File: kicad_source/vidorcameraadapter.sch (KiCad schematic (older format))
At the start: 67 parts, among them CN1 TE_2041119-2, CN2 RS2-20-G, CN3 DNI, U1 SN74LVC2G34DBV

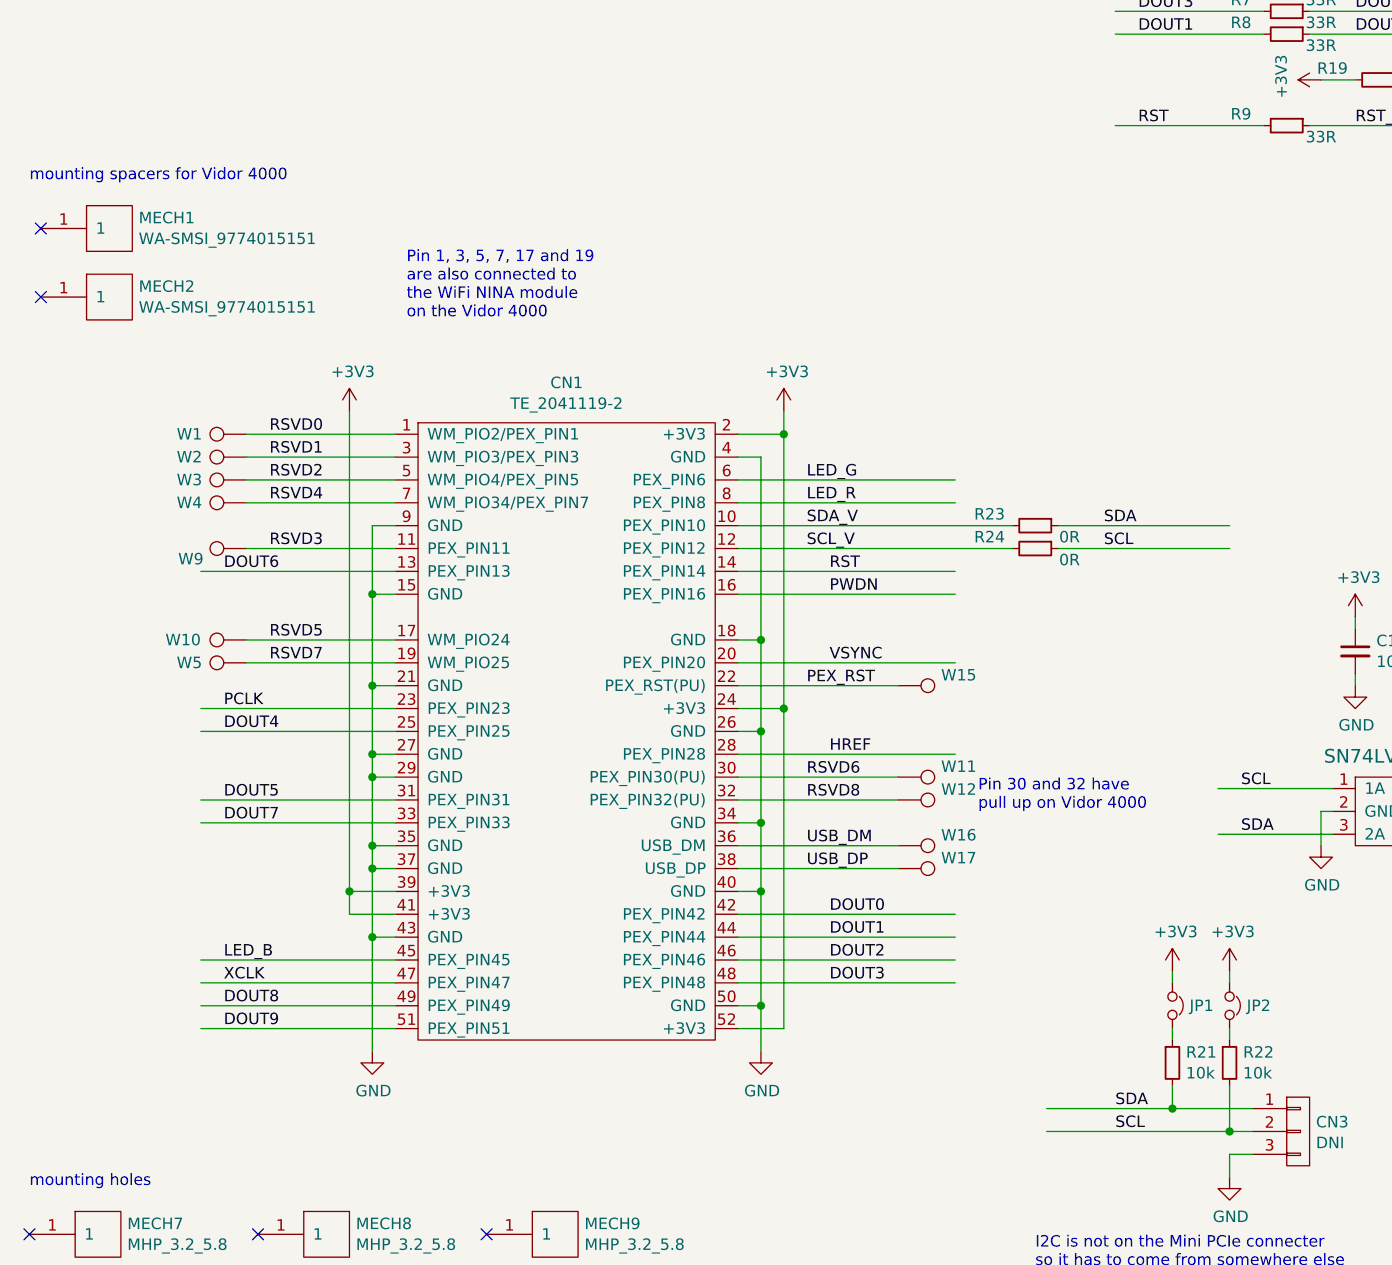
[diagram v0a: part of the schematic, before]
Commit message: restored design files from master
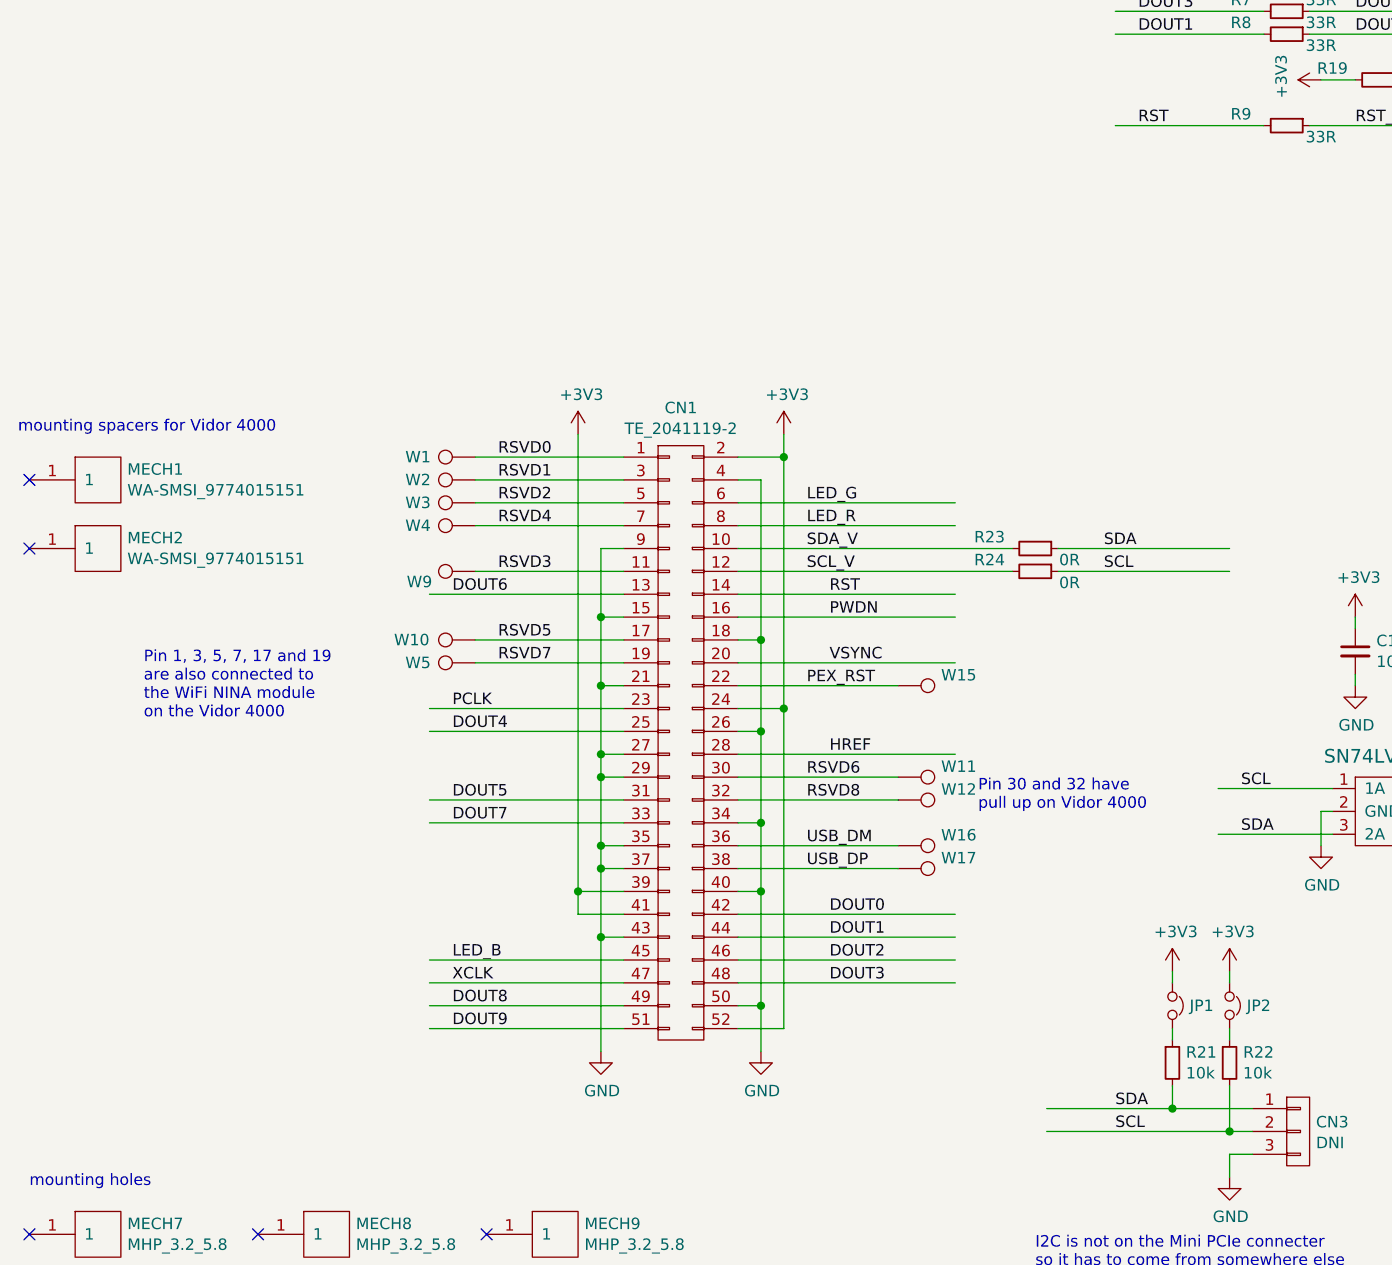
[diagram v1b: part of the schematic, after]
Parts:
- removed CN1: TE_2041119-2, connectors_pci-express:MPCIe_4mm, symbol MODULE_compute:ARDUINO_VIDOR_MPCIE
- added CN1: TE_2041119-2, connectors_pci-express:MPCIe_4mm, symbol mechanical-connectors:CONN_02X26
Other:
- moved on the sheet: MECH1, MECH2, R23, R24, W1, W10, W2, W3, W4, W5, W9
